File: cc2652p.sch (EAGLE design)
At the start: 39 parts, among them IC2 CP2102, J3 CORTEX_DEBUG_SMD, J5 TYPE-C-31-M-12, Q1 SI2323DS, U1 MCP73831, U2 ap2112k-3.3, U3 XC61CN3202MR-G

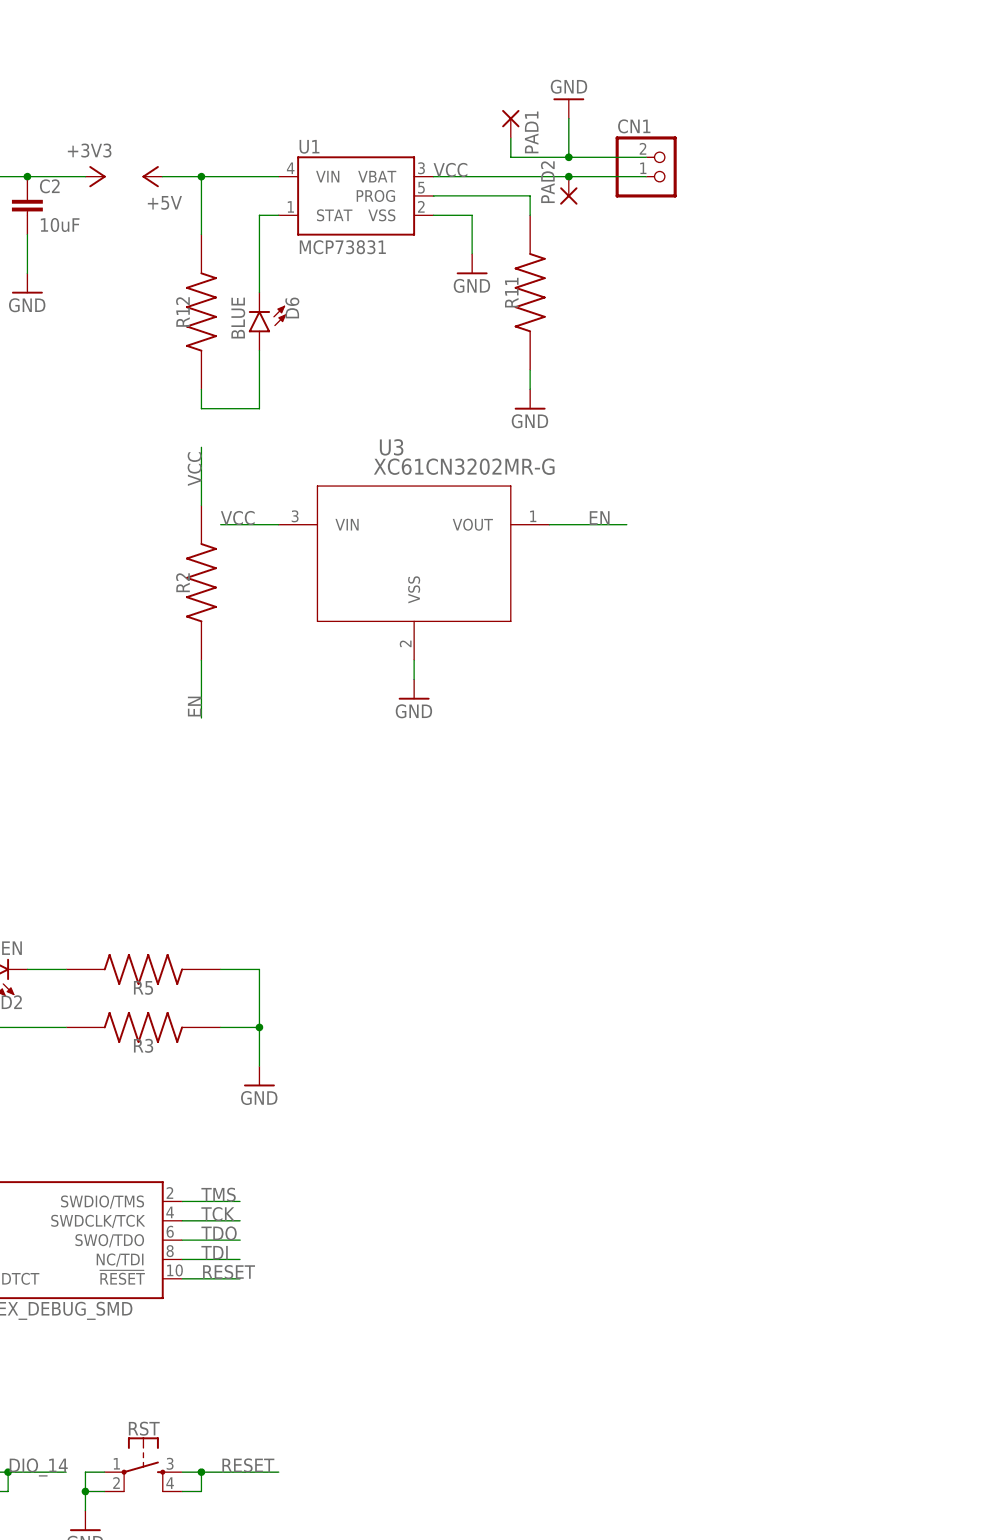
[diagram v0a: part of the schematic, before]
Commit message: Add files via upload
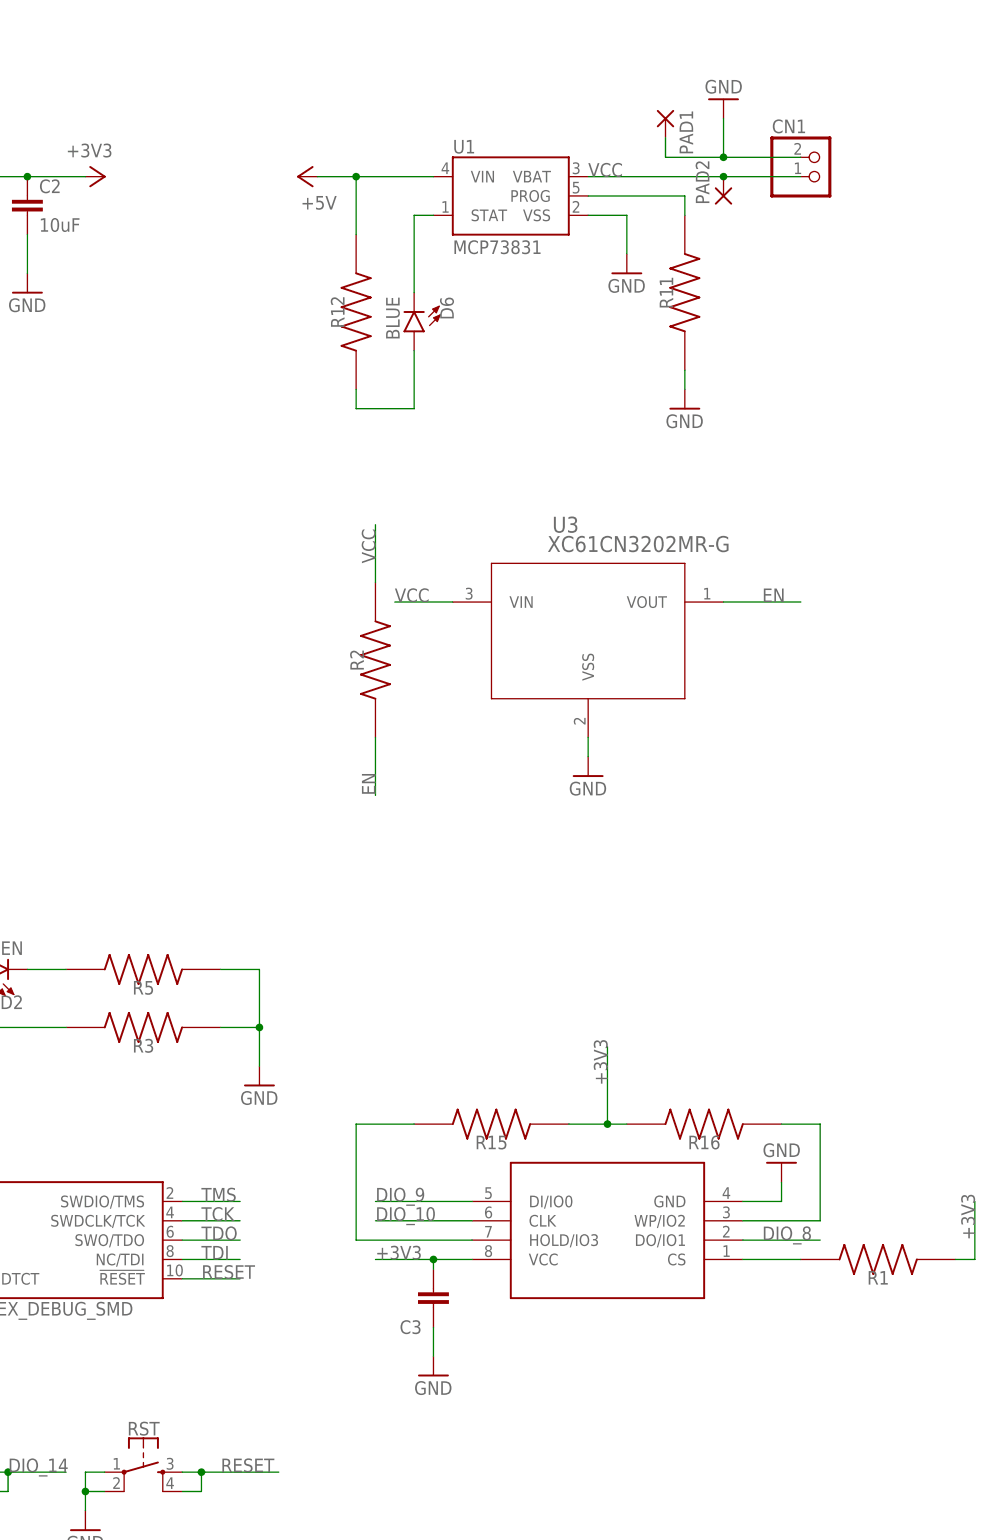
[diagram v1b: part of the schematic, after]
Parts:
- added C3: 100n, discretes-dev:CAP0402
- added R1: 2.2k, RC0402FR-073M6L:RC0402FR-073M6L
- added R15, R16: 0, RC0402FR-073M6L:RC0402FR-073M6L
- added U$2: MX25R8035FM1IL0, W25Q80BVSNIG:W25Q80BVSNIG
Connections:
- new net N$12: R15.2, U$2.HOLD/IO3
- new net N$15: R16.1, U$2.WP/IO2
- new net N$17: R1.2, U$2.CS
- net +3V3: now also C3.2, R1.1, R15.1, R16.2, U$2.VCC
- net DIO_10: now also U$2.CLK
- net DIO_8: now also U$2.DO/IO1
- net DIO_9: now also U$2.DI/IO0
- net GND: now also C3.1, U$2.GND
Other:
- moved on the sheet: CN1, D6, PAD1, PAD2, R11, R12, R2, U1, U3
